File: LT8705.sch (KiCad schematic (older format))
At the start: 81 parts, among them J1 XH-2, J2 HDR-M-2.54-1*4P, Q1 CSD19532Q5B, Q2 CSD19532Q5B, Q3 NC, Q4 NC, Q5 NC, Q6 NC, Q7 CSD19532Q5B, Q8 CSD19532Q5B, U1 LT8705EFE

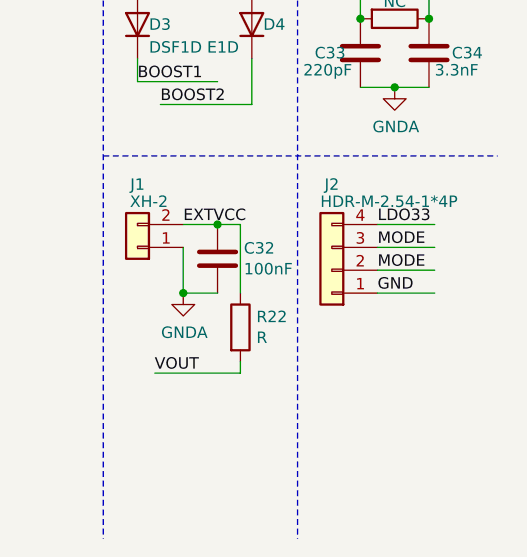
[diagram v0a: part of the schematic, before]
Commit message: 1
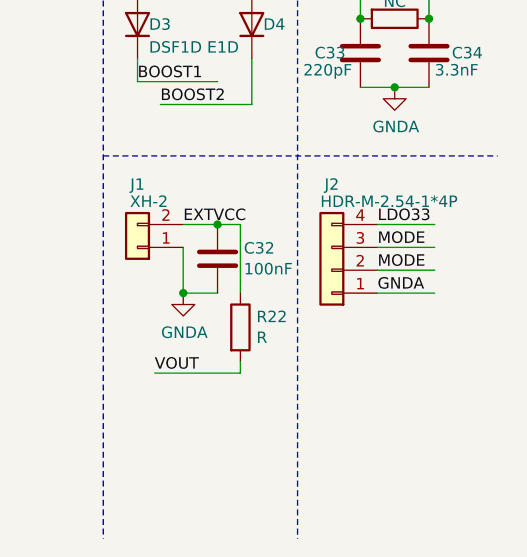
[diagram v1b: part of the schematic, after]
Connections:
- net labels removed: GND
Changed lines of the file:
@@
 MODE
 Text Label 10700 5450 0    50   ~ 0
-GND
+GNDA
 $Comp
 L LT8705-rescue:GNDA-power #PWR03
